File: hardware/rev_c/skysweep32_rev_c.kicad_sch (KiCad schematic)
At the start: 99 parts, among them J1 USB4105-GF-A, J2 Molex 104031-0811, J3 OLED STEMMA QT, J4 OPTIONAL VIBRATION MOTOR, J5 SUB-GHZ SMA, J6 BATTERY — ADAFRUIT PID 328, J7 5.8-GHZ SMA, Q1 AO3400A, Q2 AO3400A, SW1 RESET, SW2 BOOT, SW3 USER, SW4 SYSTEM POWER, U1 ESP32-S3-WROOM-1-N16R8, U2 USBLC6-2SC6, U3 AP63203WU-7, U4 BQ24074RGTR, U5 TPS61232DRCR, U6 MAX17048G+T10

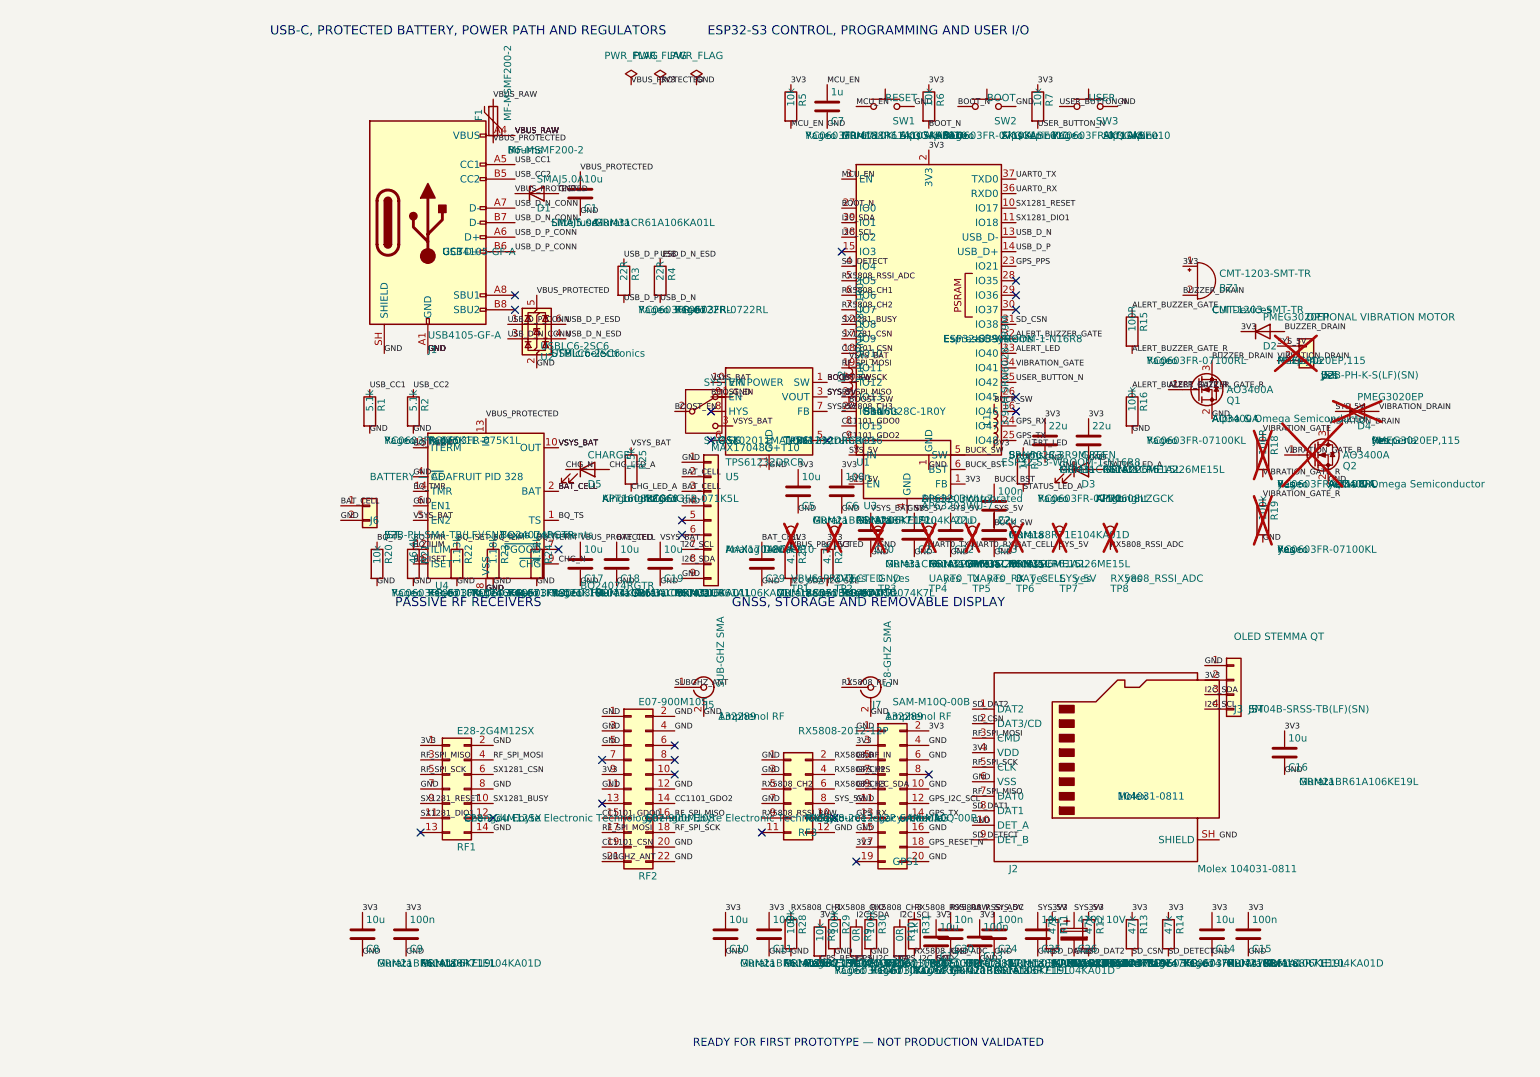
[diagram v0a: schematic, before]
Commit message: hardware: publish reviewed Rev C engineering package
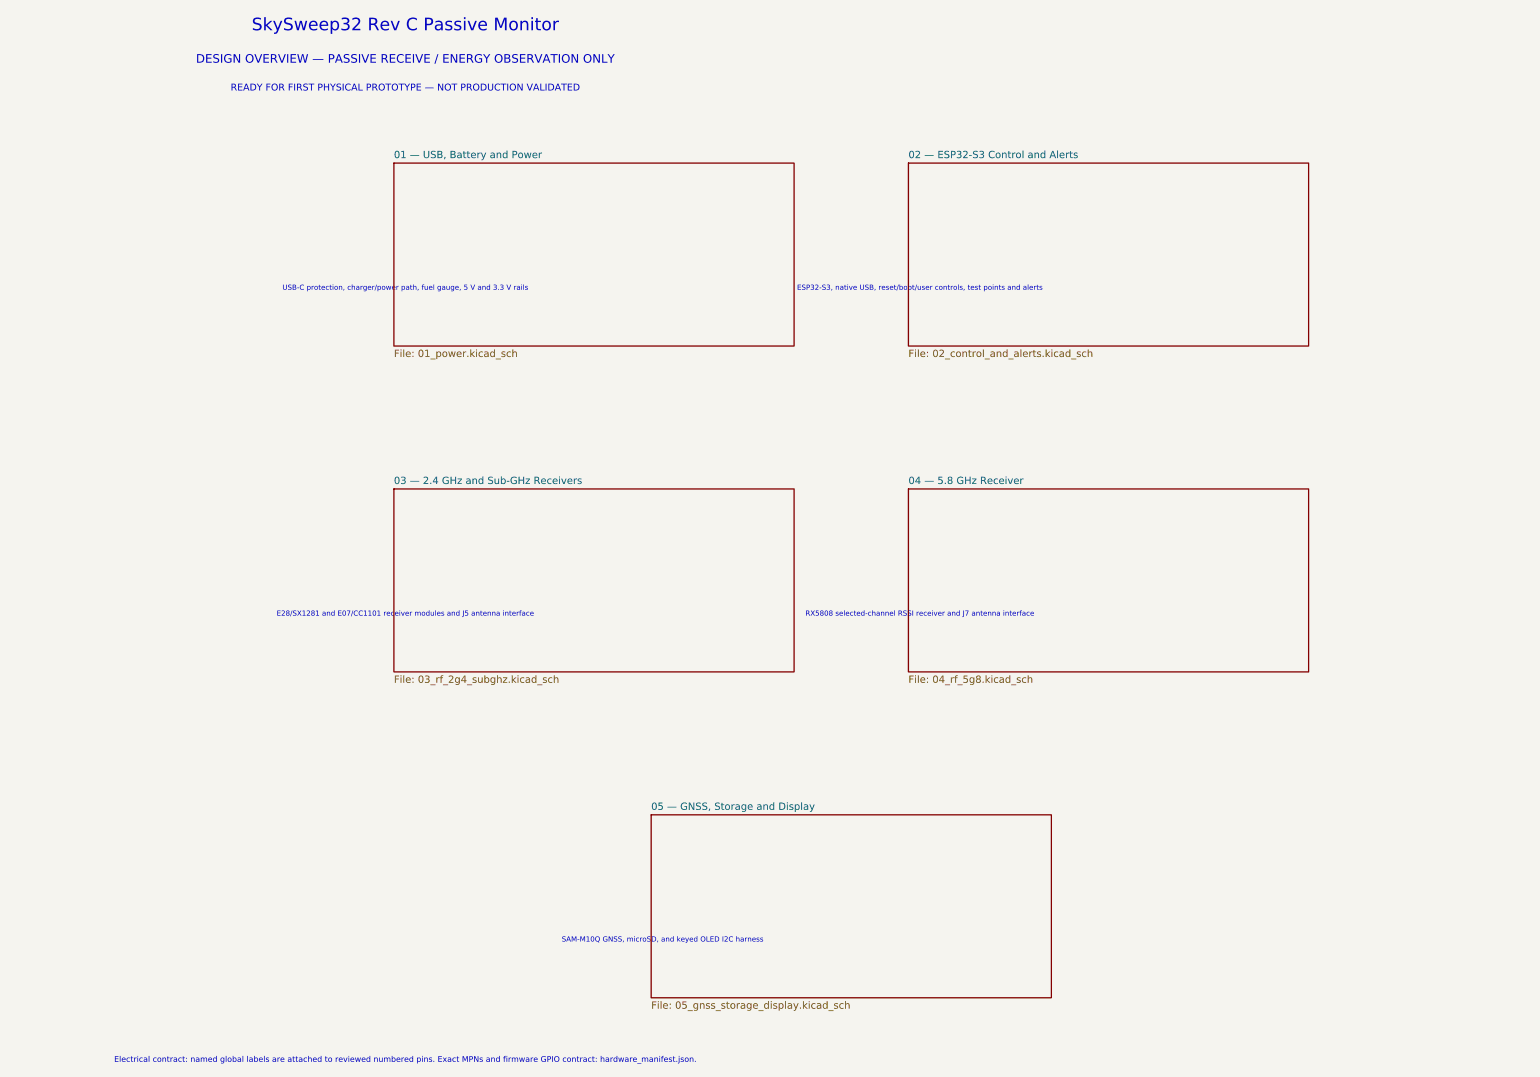
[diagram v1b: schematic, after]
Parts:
- removed BZ1: CMT-1203-SMT-TR, SkySweep32RevC:Buzzer_CUI_CMT_1203_SMT_TR, symbol Device:Buzzer
- removed C1, C17, C18, C19: 10u, Capacitor_SMD:C_1206_3216Metric, symbol Device:C
- removed C10, C12, C14, C16, C25, C5, C8: 10u, Capacitor_SMD:C_0805_2012Metric, symbol Device:C
- removed C11, C13, C15, C2, C24, C29, C6, C9: 100n, Capacitor_SMD:C_0603_1608Metric, symbol Device:C
- removed C20, C21, C22, C23, C3, C4: 22u, Capacitor_SMD:C_1206_3216Metric, symbol Device:C
- removed C26: 470u 10V, Capacitor_SMD:CP_Elec_10x10, symbol Device:C_Polarized
- removed C30: 10n, Capacitor_SMD:C_0603_1608Metric, symbol Device:C
- removed C7: 1u, Capacitor_SMD:C_0603_1608Metric, symbol Device:C
- removed D1: SMAJ5.0A, Diode_SMD:D_SMA, symbol Device:D_Zener
- removed D2, D4: PMEG3020EP, Diode_SMD:D_SOD-128, symbol Device:D
- removed D3: GREEN, LED_SMD:LED_0603_1608Metric, symbol Device:LED
- removed D5: CHARGE, LED_SMD:LED_0603_1608Metric, symbol Device:LED
- removed F1: MF-MSMF200-2, Fuse:Fuse_1812_4532Metric, symbol Device:Polyfuse
- removed GPS1: SAM-M10Q-00B, SkySweep32RevC:Module_UBlox_SAM_M10Q, symbol Connector_Generic:Conn_02x10_Odd_Even
- removed J1: USB4105-GF-A, Connector_USB:USB_C_Receptacle_GCT_USB4105-xx-A_16P_TopMnt_Horizontal, symbol Connector:USB_C_Receptacle_USB2.0_16P
- removed J2: Molex 104031-0811, Connector_Card:microSD_HC_Molex_104031-0811, symbol Connector:Micro_SD_Card_Det2
- removed J3: OLED STEMMA QT, Connector_JST:JST_SH_SM04B-SRSS-TB_1x04-1MP_P1.00mm_Horizontal, symbol Connector_Generic:Conn_01x04
- removed J4: OPTIONAL VIBRATION MOTOR, Connector_JST:JST_PH_B2B-PH-K_1x02_P2.00mm_Vertical, symbol Connector_Generic:Conn_01x02
- removed J5: SUB-GHZ SMA, Connector_Coaxial:SMA_Amphenol_132289_EdgeMount, symbol Connector:Conn_Coaxial
- removed J6: BATTERY — ADAFRUIT PID 328, Connector_JST:JST_PH_S2B-PH-SM4-TB_1x02-1MP_P2.00mm_Horizontal, symbol Connector_Generic:Conn_01x02
- removed J7: 5.8-GHZ SMA, Connector_Coaxial:SMA_Amphenol_132289_EdgeMount, symbol Connector:Conn_Coaxial
- removed L1: 3.9uH SRN6028-3R9M, Inductor_SMD:L_Bourns-SRN6028, symbol Device:L
- removed L2: 1uH SRN6028C-1R0Y, Inductor_SMD:L_Bourns-SRN6028, symbol Device:L
- removed Q1, Q2: AO3400A, Package_TO_SOT_SMD:SOT-23, symbol Transistor_FET:Q_NMOS_GSD
- removed R1, R2: 5.1k, Resistor_SMD:R_0603_1608Metric, symbol Device:R
- removed R10, R9: 0R, Resistor_SMD:R_0603_1608Metric, symbol Device:R
- removed R11, R12, R13, R14: 47k, Resistor_SMD:R_0603_1608Metric, symbol Device:R
- removed R15, R18: 100R, Resistor_SMD:R_0603_1608Metric, symbol Device:R
- removed R16, R19, R28, R29, R30: 100k, Resistor_SMD:R_0603_1608Metric, symbol Device:R
- removed R17, R31: 1k, Resistor_SMD:R_0603_1608Metric, symbol Device:R
- removed R20, R5, R6, R7, R8: 10k, Resistor_SMD:R_0603_1608Metric, symbol Device:R
- removed R21: 46.4k, Resistor_SMD:R_0603_1608Metric, symbol Device:R
- removed R22: 1.13k, Resistor_SMD:R_0603_1608Metric, symbol Device:R
- removed R23: 1.18k, Resistor_SMD:R_0603_1608Metric, symbol Device:R
- removed R24: 4.12k, Resistor_SMD:R_0603_1608Metric, symbol Device:R
- removed R25: 1.5k, Resistor_SMD:R_0603_1608Metric, symbol Device:R
- removed R26, R27: 4.7k, Resistor_SMD:R_0603_1608Metric, symbol Device:R
- removed R3, R4: 22R, Resistor_SMD:R_0603_1608Metric, symbol Device:R
- removed RF1: E28-2G4M12SX, SkySweep32RevC:Module_Ebyte_E28_2G4M12SX, symbol Connector_Generic:Conn_02x07_Odd_Even
- removed RF2: E07-900M10S, SkySweep32RevC:Module_Ebyte_E07_900M10S, symbol Connector_Generic:Conn_02x11_Odd_Even
- removed RF3: RX5808-2012-12P, SkySweep32RevC:Module_RX5808_2012_12P, symbol Connector_Generic:Conn_02x06_Odd_Even
- removed SW1: RESET, Button_Switch_SMD:SW_SPST_SKQG_WithoutStem, symbol Switch:SW_Push
- removed SW2: BOOT, Button_Switch_SMD:SW_SPST_SKQG_WithoutStem, symbol Switch:SW_Push
- removed SW3: USER, Button_Switch_SMD:SW_SPST_SKQG_WithoutStem, symbol Switch:SW_Push
- removed SW4: SYSTEM POWER, Button_Switch_THT:SW_Slide_SPDT_Angled_CK_OS102011MA1Q, symbol Switch:SW_SPDT
- removed TP1: VBUS_PROTECTED, TestPoint:TestPoint_Pad_D1.0mm, symbol Connector:TestPoint
- removed TP2: 3V3, TestPoint:TestPoint_Pad_D1.0mm, symbol Connector:TestPoint
- removed TP3: GND, TestPoint:TestPoint_Pad_D1.0mm, symbol Connector:TestPoint
- removed TP4: UART0_TX, TestPoint:TestPoint_Pad_D1.0mm, symbol Connector:TestPoint
- removed TP5: UART0_RX, TestPoint:TestPoint_Pad_D1.0mm, symbol Connector:TestPoint
- removed TP6: BAT_CELL, TestPoint:TestPoint_Pad_D1.0mm, symbol Connector:TestPoint
- removed TP7: SYS_5V, TestPoint:TestPoint_Pad_D1.0mm, symbol Connector:TestPoint
- removed TP8: RX5808_RSSI_ADC, TestPoint:TestPoint_Pad_D1.0mm, symbol Connector:TestPoint
- removed U1: ESP32-S3-WROOM-1-N16R8, RF_Module:ESP32-S3-WROOM-1, symbol RF_Module:ESP32-S3-WROOM-1
- removed U2: USBLC6-2SC6, Package_TO_SOT_SMD:SOT-23-6, symbol Power_Protection:USBLC6-2SC6
- removed U3: AP63203WU-7, Package_TO_SOT_SMD:TSOT-23-6, symbol Regulator_Switching:AP63203WU
- removed U4: BQ24074RGTR, Package_DFN_QFN:VQFN-16-1EP_3x3mm_P0.5mm_EP1.6x1.6mm, symbol Battery_Management:BQ24074RGT
- removed U5: TPS61232DRCR, Package_SON:Texas_S-PVSON-N10_ThermalVias, symbol Regulator_Switching:TPS61230DRC
- removed U6: MAX17048G+T10, Package_DFN_QFN:DFN-8-1EP_2x2mm_P0.5mm_EP0.9x1.3mm, symbol Connector_Generic:Conn_01x09
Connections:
- no-connect marks 25 -> 0
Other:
- added sheet 01 — USB, Battery and Power (01_power.kicad_sch)
- added sheet 02 — ESP32-S3 Control and Alerts (02_control_and_alerts.kicad_sch)
- added sheet 03 — 2.4 GHz and Sub-GHz Receivers (03_rf_2g4_subghz.kicad_sch)
- added sheet 04 — 5.8 GHz Receiver (04_rf_5g8.kicad_sch)
- added sheet 05 — GNSS, Storage and Display (05_gnss_storage_display.kicad_sch)
- note added: "DESIGN OVERVIEW — PASSIVE RECEIVE / ENERGY OBSERVATION ONLY"
- note added: "E28/SX1281 and E07/CC1101 receiver modules and J5 antenna interface"
- note added: "ESP32-S3, native USB, reset/boot/user controls, test points and alerts"
- note added: "Electrical contract: named global labels are attached to reviewed numbered pins. Exact MPNs and firmware GPIO contract: hardware_manifest.json."
- note added: "READY FOR FIRST PHYSICAL PROTOTYPE — NOT PRODUCTION VALIDATED"
- note added: "RX5808 selected-channel RSSI receiver and J7 antenna interface"
- note added: "SAM-M10Q GNSS, microSD, and keyed OLED I2C harness"
- note added: "SkySweep32 Rev C Passive Monitor"
- note added: "USB-C protection, charger/power path, fuel gauge, 5 V and 3.3 V rails"
- note removed: "ESP32-S3 CONTROL, PROGRAMMING AND USER I/O"
- note removed: "GNSS, STORAGE AND REMOVABLE DISPLAY"
- note removed: "PASSIVE RF RECEIVERS"
- note removed: "READY FOR FIRST PROTOTYPE — NOT PRODUCTION VALIDATED"
- note removed: "USB-C, PROTECTED BATTERY, POWER PATH AND REGULATORS"
